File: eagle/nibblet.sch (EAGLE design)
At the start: 35 parts, among them IC1 MEGA8-AI

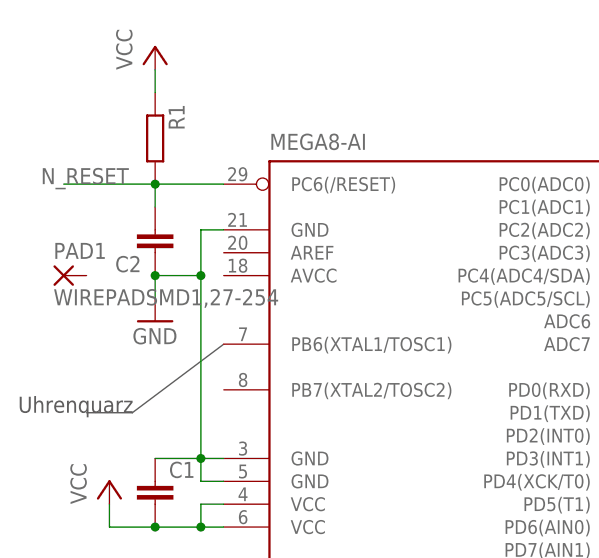
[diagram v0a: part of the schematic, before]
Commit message: pad for battery. GND on the PCB??
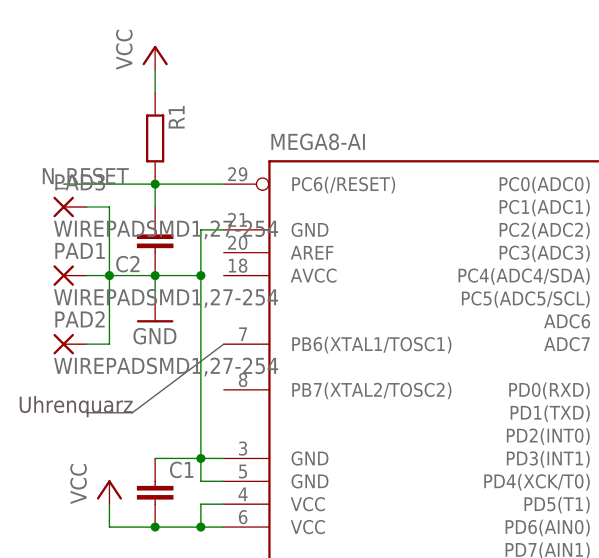
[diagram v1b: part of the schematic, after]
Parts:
- added PAD2, PAD3: WIREPADSMD1,27-254, wirepad:WIREPADSMD1,27-254
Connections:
- net GND: now also PAD1.P, PAD2.P, PAD3.P
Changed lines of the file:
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@@
 <?xml version="1.0" encoding="utf-8"?>
 <!DOCTYPE eagle SYSTEM "eagle.dtd">
-<eagle version="6.4">
+<eagle version="6.5.0">
 <drawing>
 <settings>
@@
 <part name="R14" library="rcl" deviceset="R-EU_" device="R0805"/>
 <part name="R15" library="rcl" deviceset="R-EU_" device="R0805"/>
+<part name="PAD2" library="wirepad" deviceset="WIREPAD" device="SMD1,27-254"/>
+<part name="PAD3" library="wirepad" deviceset="WIREPAD" device="SMD1,27-254"/>
 </parts>
 <sheets>
@@
 <instance part="R14" gate="G$1" x="78.74" y="86.36"/>
 <instance part="R15" gate="G$1" x="78.74" y="83.82"/>
+<instance part="PAD2" gate="G$1" x="5.08" y="78.74"/>
+<instance part="PAD3" gate="G$1" x="5.08" y="93.98"/>
 </instances>
 <busses>
@@
 <pinref part="C1" gate="G$1" pin="1"/>
 <pinref part="C2" gate="G$1" pin="1"/>
-</segment>
-<segment>
+<pinref part="PAD1" gate="G$1" pin="P"/>
+<wire x1="15.24" y1="86.36" x2="10.16" y2="86.36" width="0.1524" layer="91"/>
+<pinref part="PAD3" gate="G$1" pin="P"/>
+<wire x1="10.16" y1="86.36" x2="7.62" y2="86.36" width="0.1524" layer="91"/>
+<wire x1="7.62" y1="93.98" x2="10.16" y2="93.98" width="0.1524" layer="91"/>
+<wire x1="10.16" y1="93.98" x2="10.16" y2="86.36" width="0.1524" layer="91"/>
+<junction x="10.16" y="86.36"/>
+<wire x1="10.16" y1="86.36" x2="10.16" y2="78.74" width="0.1524" layer="91"/>
+<pinref part="PAD2" gate="G$1" pin="P"/>
+<wire x1="10.16" y1="78.74" x2="7.62" y2="78.74" width="0.1524" layer="91"/>
+</segment>
+<segment>

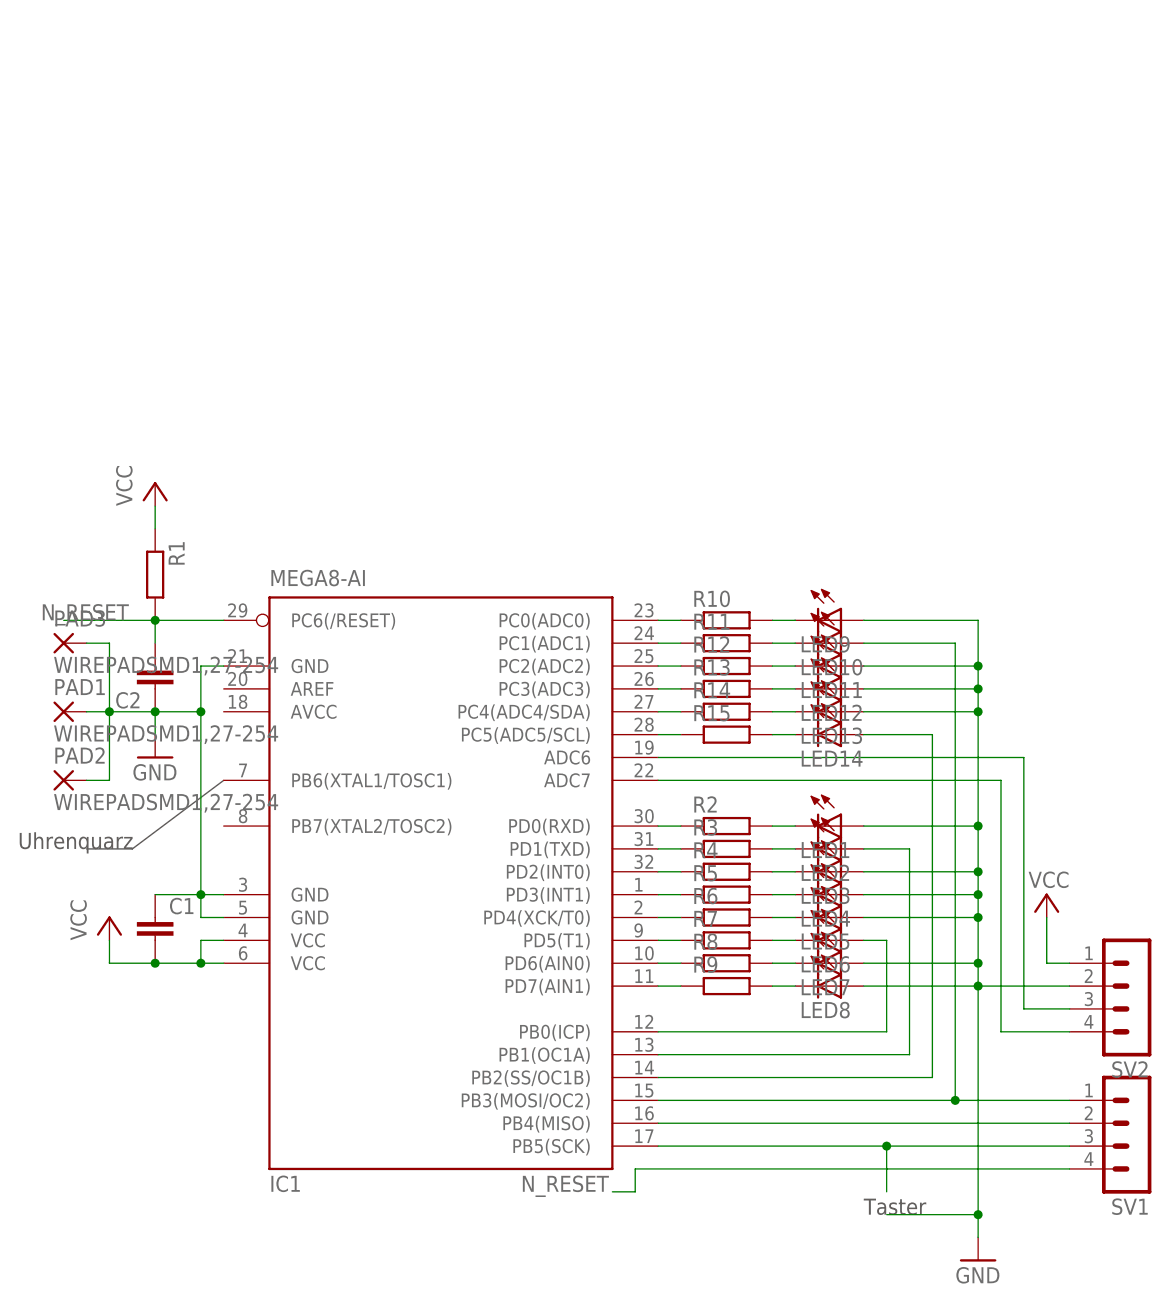
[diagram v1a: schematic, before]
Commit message: pin checking, LED array
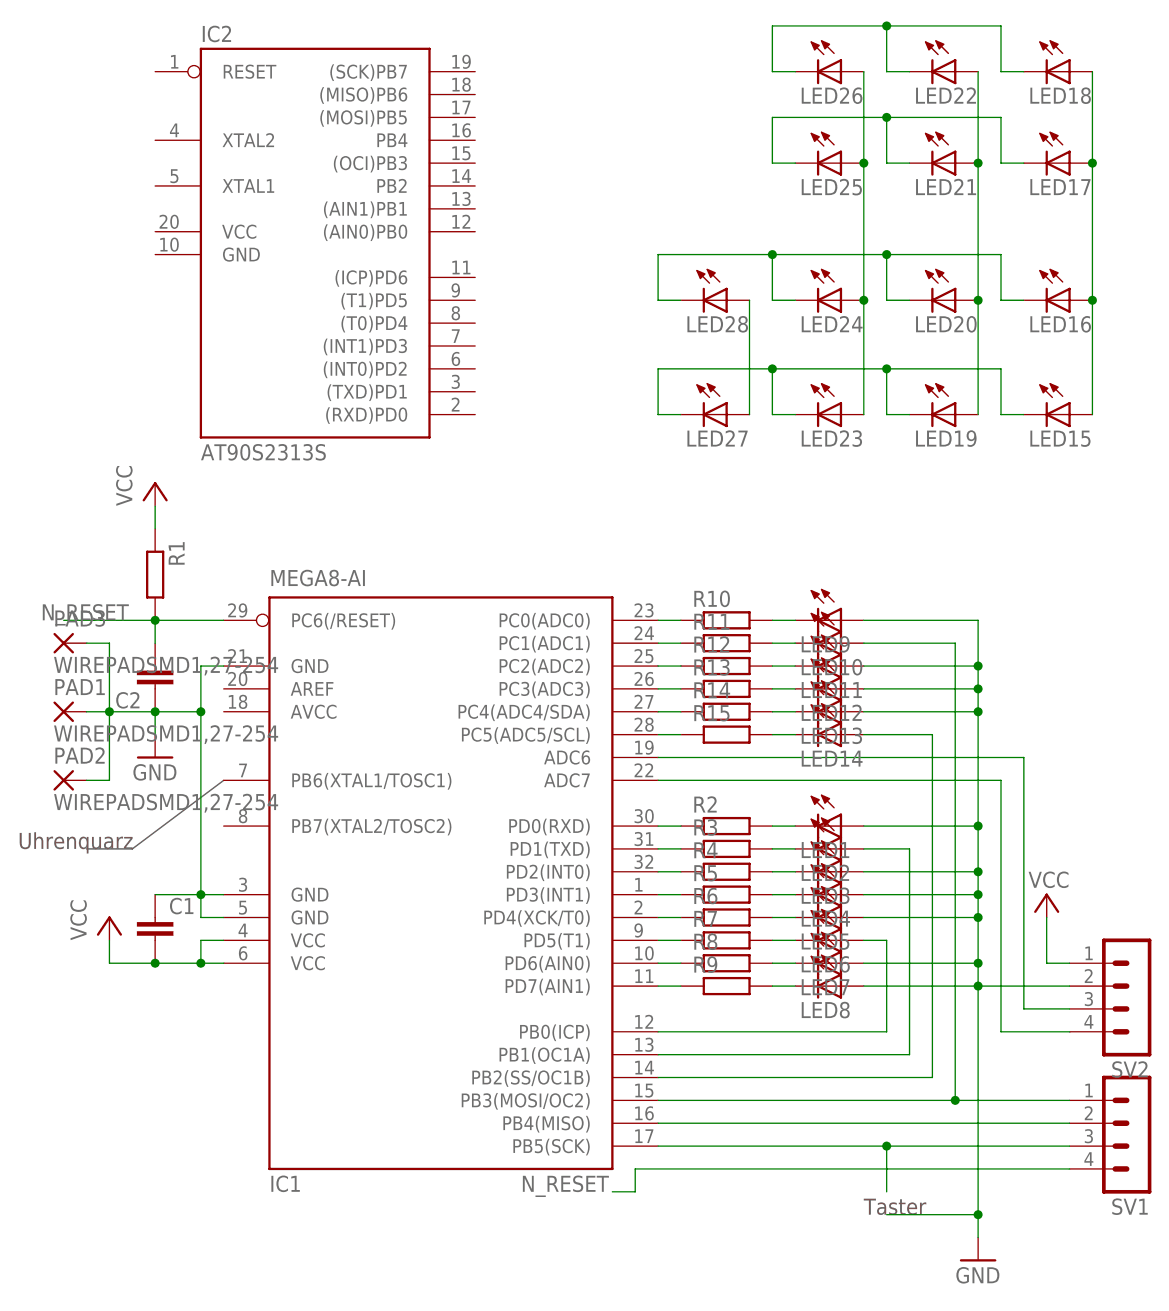
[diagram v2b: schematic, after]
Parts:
- added IC2: AT90S2313S, atmel:AT90S2313S
- added LED15, LED16, LED17, LED18, LED19, LED20, LED21, LED22, LED23, LED24, LED25, LED26, LED27, LED28: (no value), led:LEDCHIP-LED0805
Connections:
- new net N$37: LED15.C, LED19.C, LED23.C, LED27.C
- new net N$38: LED27.A, LED28.A
- new net N$39: LED23.A, LED24.A, LED25.A, LED26.A
- new net N$40: LED19.A, LED20.A, LED21.A, LED22.A
- new net N$41: LED15.A, LED16.A, LED17.A, LED18.A
- new net N$42: LED16.C, LED20.C, LED24.C, LED28.C
- new net N$43: LED17.C, LED21.C, LED25.C
- new net N$44: LED18.C, LED22.C, LED26.C
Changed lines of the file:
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@@
 <part name="PAD2" library="wirepad" deviceset="WIREPAD" device="SMD1,27-254"/>
 <part name="PAD3" library="wirepad" deviceset="WIREPAD" device="SMD1,27-254"/>
+<part name="IC2" library="atmel" deviceset="AT90S2313" device="S"/>
+<part name="LED15" library="led" deviceset="LED" device="CHIP-LED0805"/>
+<part name="LED16" library="led" deviceset="LED" device="CHIP-LED0805"/>
+<part name="LED17" library="led" deviceset="LED" device="CHIP-LED0805"/>
+<part name="LED18" library="led" deviceset="LED" device="CHIP-LED0805"/>
+<part name="LED19" library="led" deviceset="LED" device="CHIP-LED0805"/>
+<part name="LED20" library="led" deviceset="LED" device="CHIP-LED0805"/>
+<part name="LED21" library="led" deviceset="LED" device="CHIP-LED0805"/>
+<part name="LED22" library="led" deviceset="LED" device="CHIP-LED0805"/>
+<part name="LED23" library="led" deviceset="LED" device="CHIP-LED0805"/>
+<part name="LED24" library="led" deviceset="LED" device="CHIP-LED0805"/>
+<part name="LED25" library="led" deviceset="LED" device="CHIP-LED0805"/>
+<part name="LED26" library="led" deviceset="LED" device="CHIP-LED0805"/>
+<part name="LED27" library="led" deviceset="LED" device="CHIP-LED0805"/>
+<part name="LED28" library="led" deviceset="LED" device="CHIP-LED0805"/>
 </parts>
 <sheets>
@@
 <instance part="PAD2" gate="G$1" x="5.08" y="78.74"/>
 <instance part="PAD3" gate="G$1" x="5.08" y="93.98"/>
+<instance part="IC2" gate="G$1" x="33.02" y="137.16"/>
+<instance part="LED15" gate="G$1" x="116.84" y="119.38" rot="R270"/>
+<instance part="LED16" gate="G$1" x="116.84" y="132.08" rot="R270"/>
+<instance part="LED17" gate="G$1" x="116.84" y="147.32" rot="R270"/>
+<instance part="LED18" gate="G$1" x="116.84" y="157.48" rot="R270"/>
+<instance part="LED19" gate="G$1" x="104.14" y="119.38" rot="R270"/>
+<instance part="LED20" gate="G$1" x="104.14" y="132.08" rot="R270"/>
+<instance part="LED21" gate="G$1" x="104.14" y="147.32" rot="R270"/>
+<instance part="LED22" gate="G$1" x="104.14" y="157.48" rot="R270"/>
+<instance part="LED23" gate="G$1" x="91.44" y="119.38" rot="R270"/>
+<instance part="LED24" gate="G$1" x="91.44" y="132.08" rot="R270"/>
+<instance part="LED25" gate="G$1" x="91.44" y="147.32" rot="R270"/>
+<instance part="LED26" gate="G$1" x="91.44" y="157.48" rot="R270"/>
+<instance part="LED27" gate="G$1" x="78.74" y="119.38" rot="R270"/>
+<instance part="LED28" gate="G$1" x="78.74" y="132.08" rot="R270"/>
 </instances>
 <busses>
@@
 </segment>
 </net>
+<net name="N$37" class="0">
+<segment>
+<pinref part="LED27" gate="G$1" pin="C"/>
+<wire x1="73.66" y1="119.38" x2="71.12" y2="119.38" width="0.1524" layer="91"/>
+<wire x1="71.12" y1="119.38" x2="71.12" y2="124.46" width="0.1524" layer="91"/>
+<wire x1="71.12" y1="124.46" x2="83.82" y2="124.46" width="0.1524" layer="91"/>
+<wire x1="83.82" y1="124.46" x2="83.82" y2="119.38" width="0.1524" layer="91"/>
+<pinref part="LED23" gate="G$1" pin="C"/>
+<wire x1="83.82" y1="119.38" x2="86.36" y2="119.38" width="0.1524" layer="91"/>
+<wire x1="83.82" y1="124.46" x2="96.52" y2="124.46" width="0.1524" layer="91"/>
+<junction x="83.82" y="124.46"/>
+<wire x1="96.52" y1="124.46" x2="96.52" y2="119.38" width="0.1524" layer="91"/>
+<pinref part="LED19" gate="G$1" pin="C"/>
+<wire x1="96.52" y1="119.38" x2="99.06" y2="119.38" width="0.1524" layer="91"/>
+<wire x1="96.52" y1="124.46" x2="109.22" y2="124.46" width="0.1524" layer="91"/>
+<junction x="96.52" y="124.46"/>
+<wire x1="109.22" y1="124.46" x2="109.22" y2="119.38" width="0.1524" layer="91"/>
+<pinref part="LED15" gate="G$1" pin="C"/>
+<wire x1="109.22" y1="119.38" x2="111.76" y2="119.38" width="0.1524" layer="91"/>
+</segment>
+</net>
+<net name="N$38" class="0">
+<segment>
+<pinref part="LED27" gate="G$1" pin="A"/>
+<pinref part="LED28" gate="G$1" pin="A"/>
+<wire x1="81.28" y1="119.38" x2="81.28" y2="132.08" width="0.1524" layer="91"/>
+</segment>
+</net>
+<net name="N$39" class="0">
+<segment>
+<pinref part="LED23" gate="G$1" pin="A"/>
+<pinref part="LED24" gate="G$1" pin="A"/>
+<wire x1="93.98" y1="119.38" x2="93.98" y2="132.08" width="0.1524" layer="91"/>
+<pinref part="LED25" gate="G$1" pin="A"/>
+<wire x1="93.98" y1="132.08" x2="93.98" y2="147.32" width="0.1524" layer="91"/>
+<junction x="93.98" y="132.08"/>
+<pinref part="LED26" gate="G$1" pin="A"/>
+<wire x1="93.98" y1="147.32" x2="93.98" y2="157.48" width="0.1524" layer="91"/>
+<junction x="93.98" y="147.32"/>
+</segment>
+</net>
+<net name="N$40" class="0">
+<segment>
+<pinref part="LED19" gate="G$1" pin="A"/>
+<pinref part="LED20" gate="G$1" pin="A"/>
+<wire x1="106.68" y1="119.38" x2="106.68" y2="132.08" width="0.1524" layer="91"/>
+<pinref part="LED21" gate="G$1" pin="A"/>
+<wire x1="106.68" y1="132.08" x2="106.68" y2="147.32" width="0.1524" layer="91"/>
+<junction x="106.68" y="132.08"/>
+<pinref part="LED22" gate="G$1" pin="A"/>
+<wire x1="106.68" y1="147.32" x2="106.68" y2="157.48" width="0.1524" layer="91"/>
+<junction x="106.68" y="147.32"/>
+</segment>
+</net>
+<net name="N$41" class="0">
+<segment>
+<pinref part="LED15" gate="G$1" pin="A"/>
+<pinref part="LED16" gate="G$1" pin="A"/>
+<wire x1="119.38" y1="119.38" x2="119.38" y2="132.08" width="0.1524" layer="91"/>
+<pinref part="LED17" gate="G$1" pin="A"/>
+<wire x1="119.38" y1="132.08" x2="119.38" y2="147.32" width="0.1524" layer="91"/>
+<junction x="119.38" y="132.08"/>
+<pinref part="LED18" gate="G$1" pin="A"/>
+<wire x1="119.38" y1="147.32" x2="119.38" y2="157.48" width="0.1524" layer="91"/>
+<junction x="119.38" y="147.32"/>
+</segment>
+</net>
+<net name="N$42" class="0">
+<segment>
+<pinref part="LED28" gate="G$1" pin="C"/>
+<wire x1="73.66" y1="132.08" x2="71.12" y2="132.08" width="0.1524" layer="91"/>
+<wire x1="71.12" y1="132.08" x2="71.12" y2="137.16" width="0.1524" layer="91"/>
+<wire x1="71.12" y1="137.16" x2="83.82" y2="137.16" width="0.1524" layer="91"/>
+<wire x1="83.82" y1="137.16" x2="83.82" y2="132.08" width="0.1524" layer="91"/>
+<pinref part="LED24" gate="G$1" pin="C"/>
+<wire x1="83.82" y1="132.08" x2="86.36" y2="132.08" width="0.1524" layer="91"/>
+<wire x1="83.82" y1="137.16" x2="96.52" y2="137.16" width="0.1524" layer="91"/>
+<junction x="83.82" y="137.16"/>
+<wire x1="96.52" y1="137.16" x2="96.52" y2="132.08" width="0.1524" layer="91"/>
+<pinref part="LED20" gate="G$1" pin="C"/>
+<wire x1="96.52" y1="132.08" x2="99.06" y2="132.08" width="0.1524" layer="91"/>
+<wire x1="96.52" y1="137.16" x2="109.22" y2="137.16" width="0.1524" layer="91"/>
+<junction x="96.52" y="137.16"/>
+<wire x1="109.22" y1="137.16" x2="109.22" y2="132.08" width="0.1524" layer="91"/>
+<pinref part="LED16" gate="G$1" pin="C"/>
+<wire x1="109.22" y1="132.08" x2="111.76" y2="132.08" width="0.1524" layer="91"/>
+</segment>
+</net>
+<net name="N$43" class="0">
+<segment>
+<pinref part="LED25" gate="G$1" pin="C"/>
+<wire x1="86.36" y1="147.32" x2="83.82" y2="147.32" width="0.1524" layer="91"/>
+<wire x1="83.82" y1="147.32" x2="83.82" y2="152.4" width="0.1524" layer="91"/>
+<wire x1="83.82" y1="152.4" x2="96.52" y2="152.4" width="0.1524" layer="91"/>
+<wire x1="96.52" y1="152.4" x2="96.52" y2="147.32" width="0.1524" layer="91"/>
+<pinref part="LED21" gate="G$1" pin="C"/>
+<wire x1="96.52" y1="147.32" x2="99.06" y2="147.32" width="0.1524" layer="91"/>
+<wire x1="96.52" y1="152.4" x2="109.22" y2="152.4" width="0.1524" layer="91"/>
+<wire x1="109.22" y1="152.4" x2="109.22" y2="147.32" width="0.1524" layer="91"/>
+<junction x="96.52" y="152.4"/>
+<pinref part="LED17" gate="G$1" pin="C"/>
+<wire x1="109.22" y1="147.32" x2="111.76" y2="147.32" width="0.1524" layer="91"/>
+</segment>
+</net>
+<net name="N$44" class="0">
+<segment>
+<pinref part="LED26" gate="G$1" pin="C"/>
+<wire x1="86.36" y1="157.48" x2="83.82" y2="157.48" width="0.1524" layer="91"/>
+<wire x1="83.82" y1="157.48" x2="83.82" y2="162.56" width="0.1524" layer="91"/>
+<wire x1="83.82" y1="162.56" x2="96.52" y2="162.56" width="0.1524" layer="91"/>
+<wire x1="96.52" y1="162.56" x2="96.52" y2="157.48" width="0.1524" layer="91"/>
+<pinref part="LED22" gate="G$1" pin="C"/>
+<wire x1="96.52" y1="157.48" x2="99.06" y2="157.48" width="0.1524" layer="91"/>
+<wire x1="96.52" y1="162.56" x2="109.22" y2="162.56" width="0.1524" layer="91"/>
+<wire x1="109.22" y1="162.56" x2="109.22" y2="157.48" width="0.1524" layer="91"/>
+<junction x="96.52" y="162.56"/>
+<pinref part="LED18" gate="G$1" pin="C"/>
+<wire x1="109.22" y1="157.48" x2="111.76" y2="157.48" width="0.1524" layer="91"/>
+</segment>
+</net>
